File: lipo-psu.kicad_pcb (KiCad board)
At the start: 2 copper layers, 19 parts, among them J1 Conn_01x04_Female, Q1 Si2301CDS, Q2 AO3400A, Q3 Si2301CDS, U1 BQ296100, U2 TPS7A26

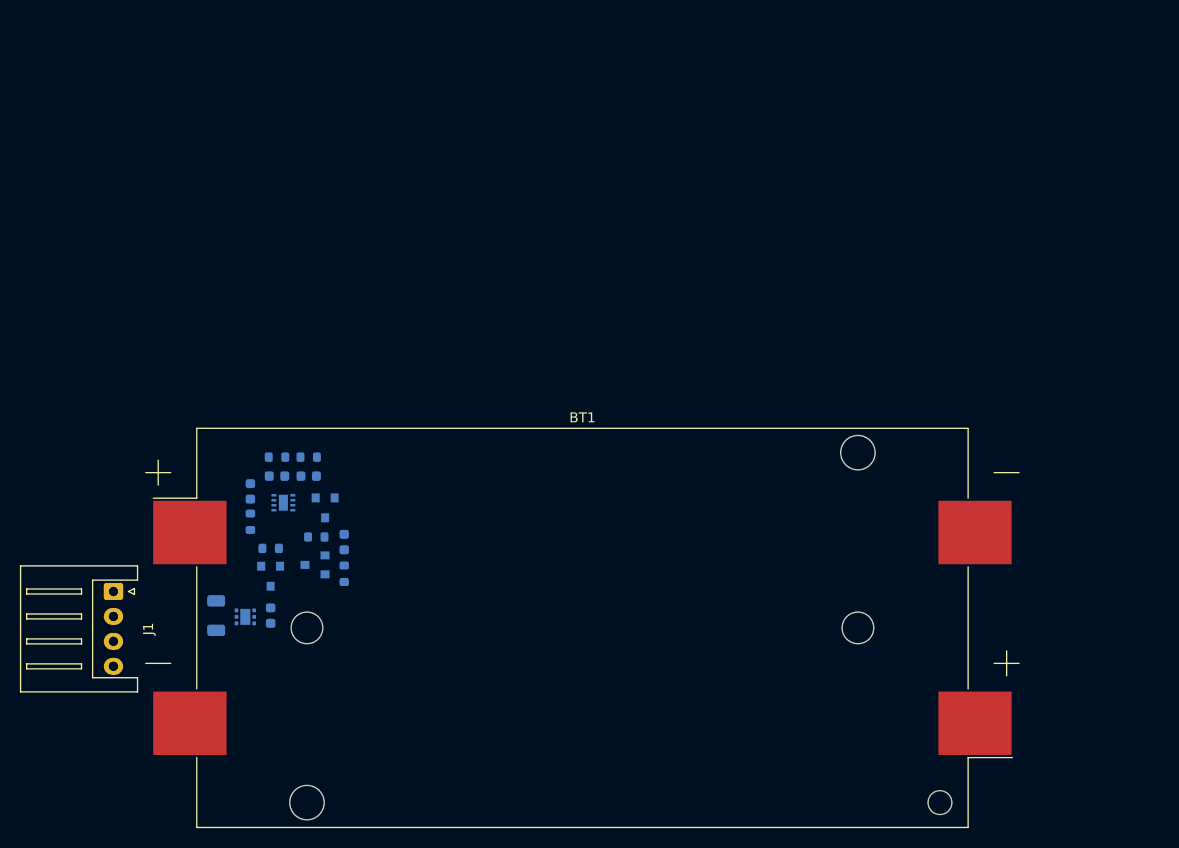
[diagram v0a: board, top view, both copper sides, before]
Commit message: changes
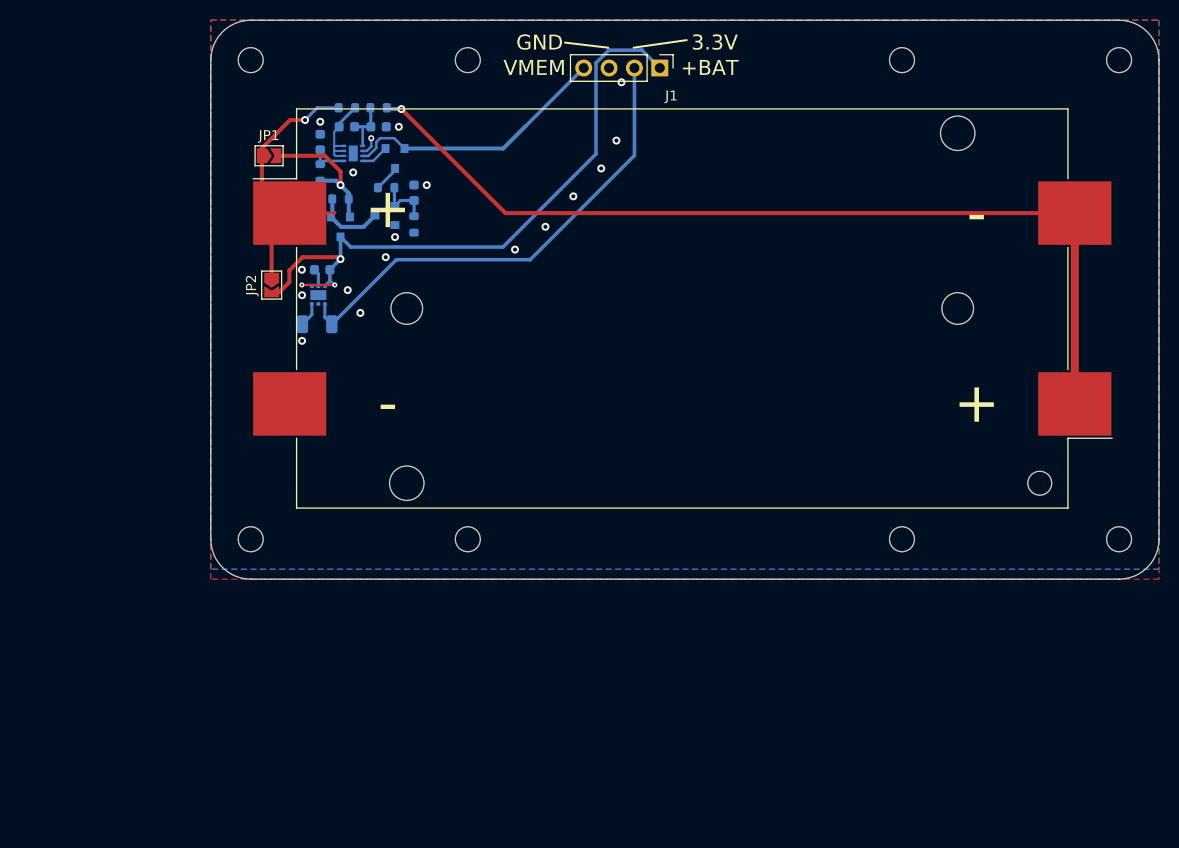
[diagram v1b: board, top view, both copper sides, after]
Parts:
- added H1: MountingHole, MountingHole:MountingHole_2.5mm, F.Cu at (109.0, 65.0)
- added H2: MountingHole, MountingHole:MountingHole_2.5mm, F.Cu at (109.0, 113.0)
- added H3: MountingHole, MountingHole:MountingHole_2.5mm, F.Cu at (196.0, 65.0)
- added H4: MountingHole, MountingHole:MountingHole_2.5mm, F.Cu at (196.0, 113.0)
- added H5: MountingHole, MountingHole:MountingHole_2.5mm, F.Cu at (130.8, 113.0)
- added H6: MountingHole, MountingHole:MountingHole_2.5mm, F.Cu at (174.2, 113.0)
- added H7: MountingHole, MountingHole:MountingHole_2.5mm, F.Cu at (130.8, 65.0)
- added H8: MountingHole, MountingHole:MountingHole_2.5mm, F.Cu at (174.2, 65.0)
- added JP1: current_test, Jumper:SolderJumper-2_P1.3mm_Open_TrianglePad1.0x1.5mm, F.Cu at (110.8, 74.6)
- added JP2: no_prot_opt, Jumper:SolderJumper-2_P1.3mm_Open_TrianglePad1.0x1.5mm, F.Cu at (111.1, 87.5)
- BT1: footprint Battery:BatteryHolder_Keystone_1048P_2x18650 -> lipo-psu:BatteryHolder_Keystone_1048P_2x18650
- J1: value Conn_01x04_Female -> 4Pin; footprint Connector_JST:JST_XH_S4B-XH-A_1x04_P2.50mm_Horizontal -> Connector_PinHeader_2.54mm:PinHeader_1x04_P2.54mm_Vertical
- R3: value 100 -> 100R
- R4: value 5 -> 4.7R
- U2: value TPS7A26 -> TPS7A2633DRVR
- moved J1 75.8 mm to (150.0, 65.8)
- moved C1 35.7 mm to (118.6, 71.7)
- moved C2 35.7 mm to (121.8, 71.7)
- moved C3 35.7 mm to (116.0, 73.2)
- moved C4 35.7 mm to (125.4, 78.3)
- moved Q1 35.7 mm to (123.5, 74.9)
- moved Q2 35.7 mm to (122.4, 80.6)
- moved Q3 35.7 mm to (118.0, 81.7)
- moved R1 35.7 mm to (118.6, 69.8)
- moved R2 35.7 mm to (121.8, 69.8)
- moved R3 35.7 mm to (116.0, 76.3)
- moved R4 35.7 mm to (122.6, 77.8)
- moved R5 35.7 mm to (125.4, 81.5)
- moved R6 35.7 mm to (118.0, 78.9)
- moved U1 35.7 mm to (119.3, 74.3)
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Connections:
- Q3 pad 2: Net-(BT1-Pad1) -> Net-(JP1-Pad2)
- R3 pad 1: Net-(BT1-Pad1) -> Net-(JP1-Pad2)
- R6 pad 2: Net-(BT1-Pad1) -> Net-(JP1-Pad2)
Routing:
- net Net-(BT1-Pad2): track 0.00 -> 92.4 mm, vias 0 -> 1
- net +BATT: track 0.00 -> 66.4 mm, vias 0 -> 3
- net +3V3: track 0.00 -> 48.4 mm
- net Net-(BT1-Pad1): track 0.00 -> 28.8 mm, vias 0 -> 1
- net VMEM: track 0.00 -> 27.0 mm
- net Net-(JP1-Pad2): track 0.00 -> 14.3 mm, vias 0 -> 1
- net Net-(C1-Pad2): track 0.00 -> 8.49 mm
- net Net-(Q2-Pad3): track 0.00 -> 7.13 mm
- net GND: track 0.00 -> 6.12 mm, vias 0 -> 18
- net Net-(C4-Pad2): track 0.00 -> 5.59 mm
- net Net-(C1-Pad1): track 0.00 -> 5.50 mm
- net Net-(C3-Pad1): track 0.00 -> 3.94 mm
- net Net-(Q1-Pad1): track 0.00 -> 2.81 mm
- net Net-(Q1-Pad3): track 0.00 -> 2.63 mm
- added copper zone on B.Cu, net GND
- added copper zone on F.Cu, net GND
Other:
- board outline added: 95 x 56 mm
- net class BAT_LINES added: clearance 0.2, trace_width 0.8128, via_dia 0.8, via_drill 0.4
- rule trace_min: 0.2 -> 0.127
- rule via_min_drill: 0.3 -> 0.2
- rule via_min_size: 0.4 -> 0.45
- board text added: "+BAT"
- board text added: "3.3V"
- board text added: "GND"
- board text added: "LiPo-PSU v1.0.0 max. 500mA"
- board text added: "VMEM"
